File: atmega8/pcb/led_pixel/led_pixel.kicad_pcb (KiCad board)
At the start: 2 copper layers, 50 x 50 mm, 61 parts, among them CON101 10PIN_ISP_AVR, IC1 ATMEGA8-AI, P1 USB_OTG, P3 CONN_01X03, P4 CONN_01X03, P5 CONN_01X04, SW1 SW_DIP_x08, U1 MC78M05CDT, U2 PT4115, U3 PT4115, U4 SN75176, U5 PT4115, Y1 CRYSTAL

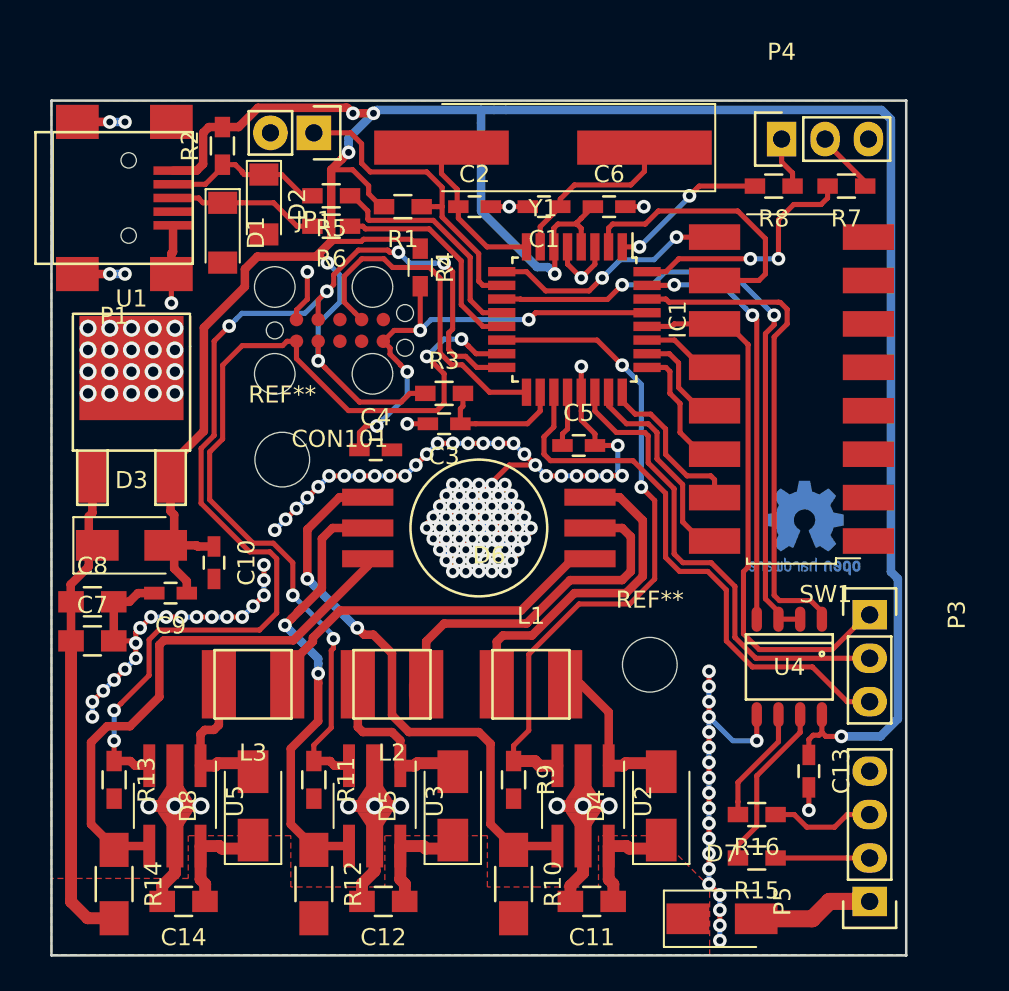
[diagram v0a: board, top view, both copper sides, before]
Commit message: finished... I hope...
replaced the ref descriptors...
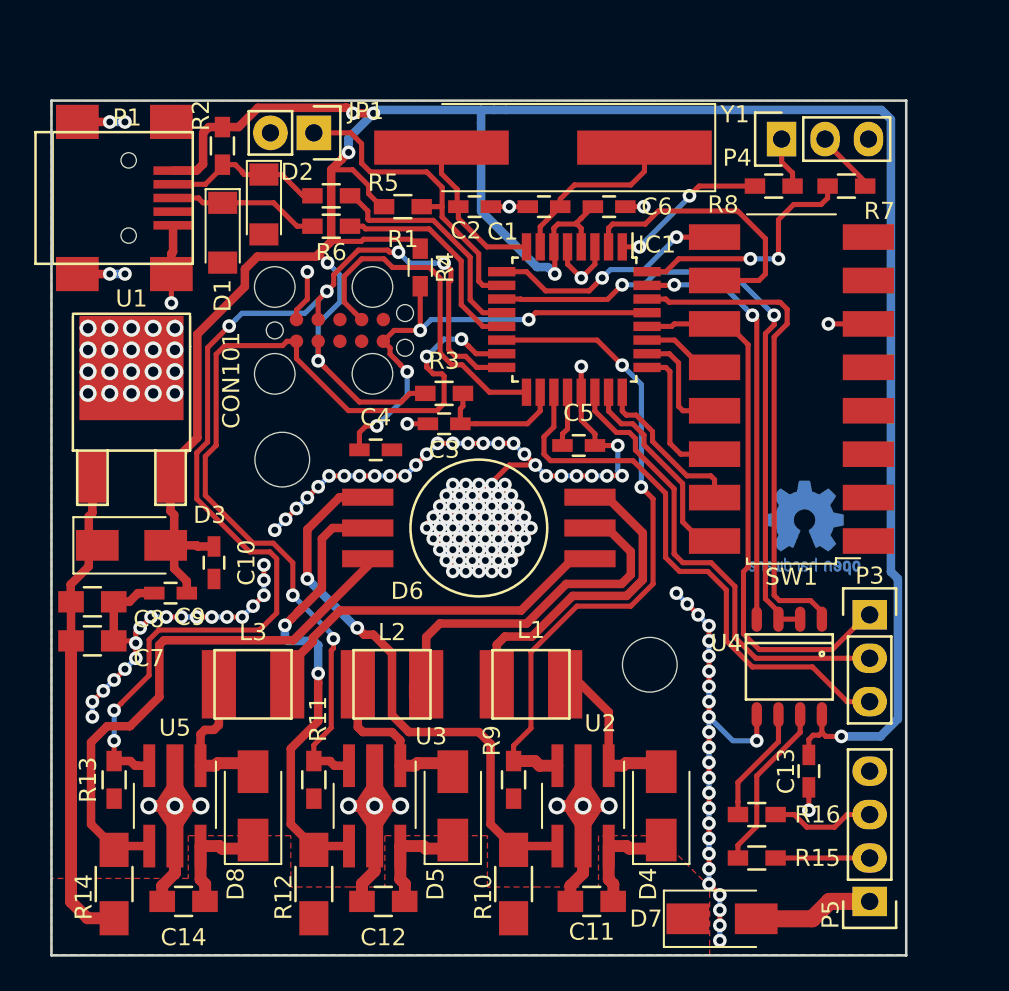
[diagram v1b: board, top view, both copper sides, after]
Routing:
- net GND: track 182.7 -> 190.4 mm, vias 169 -> 176
- net /LED_G: track 54.1 -> 55.2 mm
- net /LED_G_A: track 26.6 -> 27.5 mm
- net /DMX_2: track 7.79 -> 8.51 mm
- net /DMX_3: track 6.17 -> 6.82 mm
- net Net-(IC1-Pad22): track 28.1 -> 27.5 mm
